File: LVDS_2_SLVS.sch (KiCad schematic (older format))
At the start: 6 parts

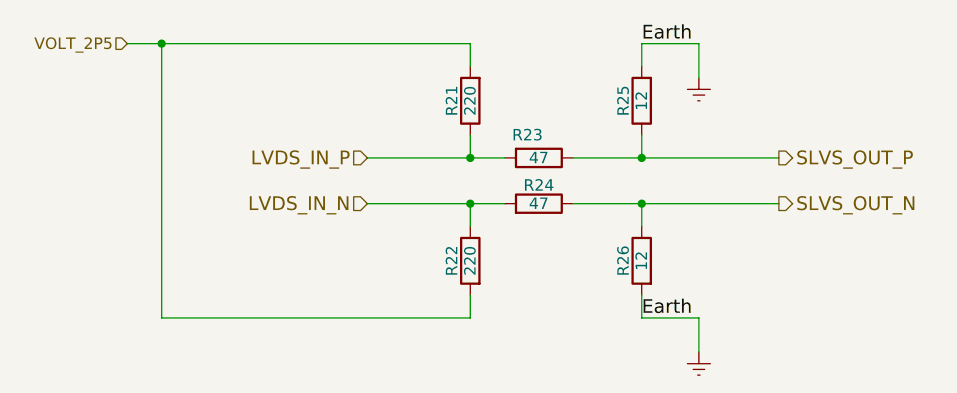
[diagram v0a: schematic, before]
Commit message: before re-arranging
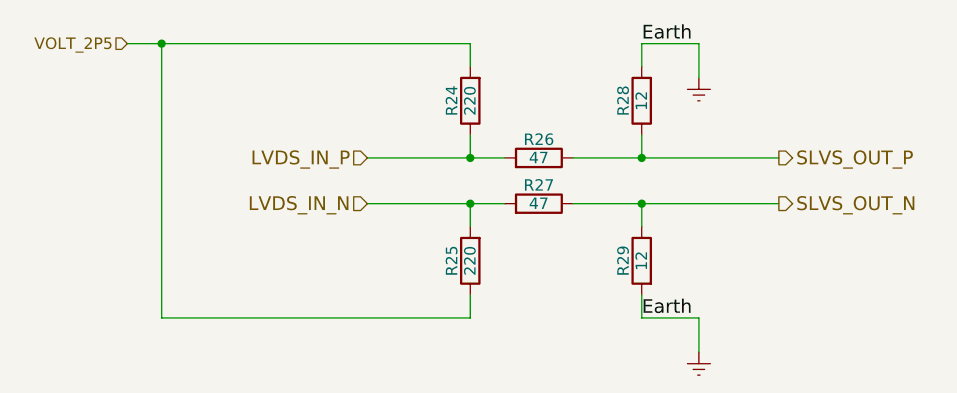
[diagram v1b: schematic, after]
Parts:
- removed R98: 220, Resistors_SMD:R_0805, symbol Device:R
- removed R99: 47, Resistors_SMD:R_0805, symbol Device:R
- added R13: 220, Resistors_SMD:R_0603, symbol Device:R
- added R14: 47, Resistors_SMD:R_0603, symbol Device:R
- R12: renamed from R97; footprint Resistors_SMD:R_0805 -> Resistors_SMD:R_0603; Part Number RC0805FR-07220RL -> RC0603FR-07220RL; Power 1/8W -> 100mW
- R15: renamed from R100; footprint Resistors_SMD:R_0805 -> Resistors_SMD:R_0603; Part Number RC0805FR-0747RL -> RC0603FR-0747RL; Power 1/8W -> 100 mW
- renumbered R101 to R16, R102 to R17
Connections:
- net LVDS_IN_N: now also R13.2
- net LVDS_IN_P: now also R14.2
- net SLVS_OUT_P: now also R14.1
- net VOLT_2P5: now also R13.1

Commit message: rev 2022
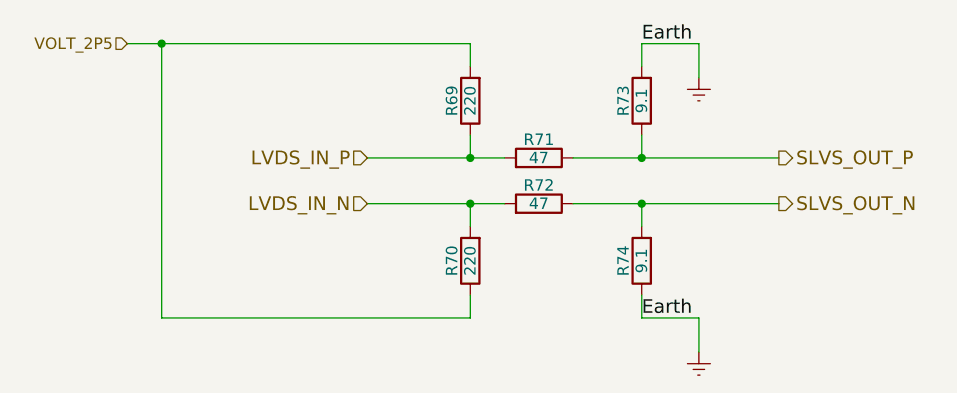
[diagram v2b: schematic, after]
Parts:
- R16, R17: value 12 -> 9.1; footprint Resistors_SMD:R_0805 -> Resistors_SMD:R_0603_HandSoldering; Part Number RC0805FR-0712RL -> (none); Power 1/8W -> 250 mW
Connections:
- net Earth: now also R17.1; no longer R17.2
- net SLVS_OUT_N: now also R17.2; no longer R17.1
